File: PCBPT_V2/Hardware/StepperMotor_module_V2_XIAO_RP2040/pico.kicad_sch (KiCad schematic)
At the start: 12 parts, among them J2 External Ctrl, U1 MOUDLE-SEEEDUINO-XIAO

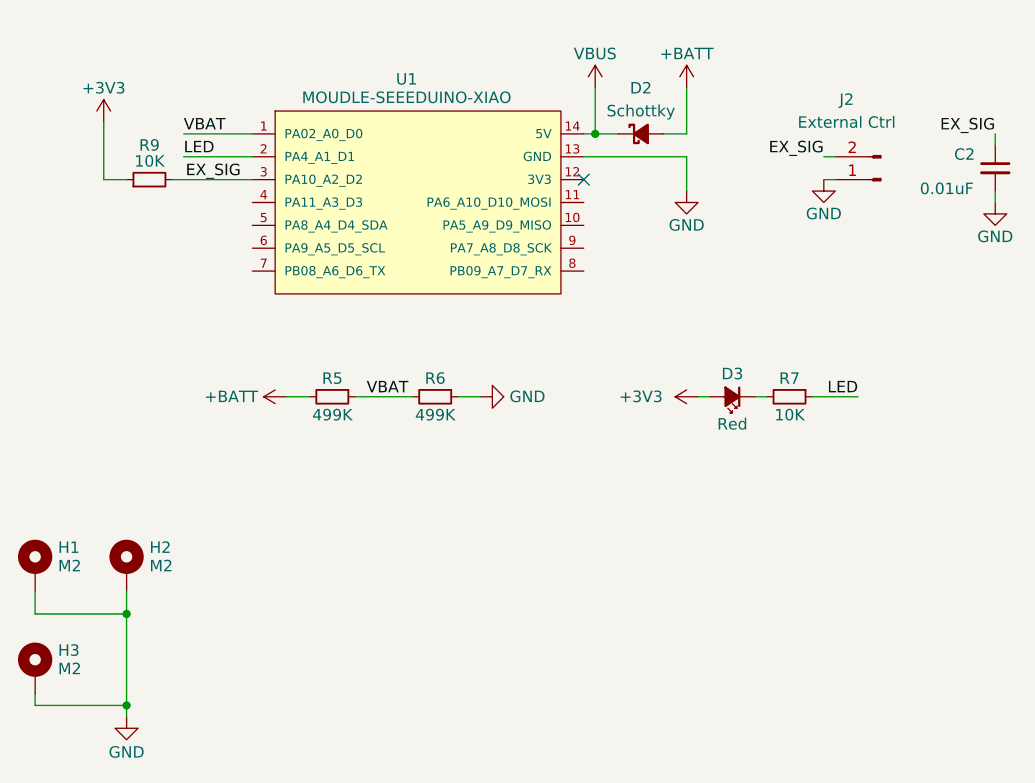
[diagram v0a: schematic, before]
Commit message: udated by FZ
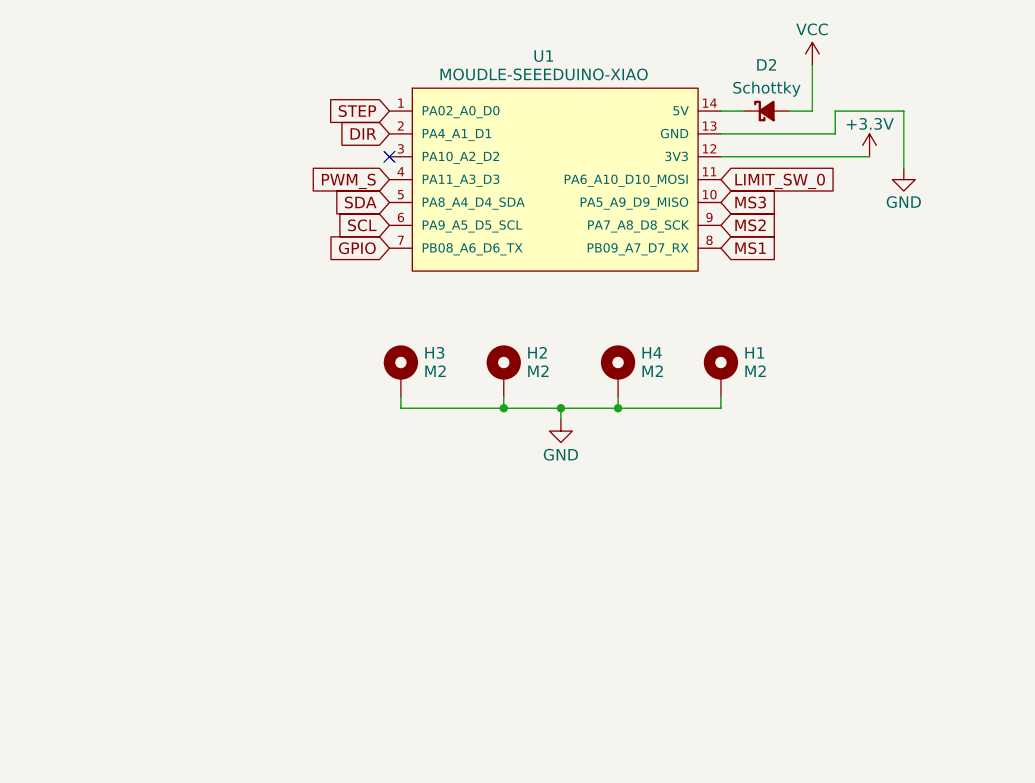
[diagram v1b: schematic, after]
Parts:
- removed C2: 0.01uF, Capacitor_SMD:C_0603_1608Metric_Pad1.08x0.95mm_HandSolder, symbol Device:C_Small
- removed D3: Red, LED_SMD:LED_0603_1608Metric_Pad1.05x0.95mm_HandSolder, symbol Device:LED_Small_Filled
- removed J2: External Ctrl, Connector_PinHeader_2.54mm:PinHeader_1x02_P2.54mm_Vertical, symbol Connector:Conn_01x02_Pin
- removed R5, R6: 499K, Resistor_SMD:R_0603_1608Metric_Pad0.98x0.95mm_HandSolder, symbol Device:R_Small
- removed R7, R9: 10K, Resistor_SMD:R_0603_1608Metric_Pad0.98x0.95mm_HandSolder, symbol Device:R_Small
- added H4: M2, MountingHole:MountingHole_2.2mm_M2_ISO7380_Pad, symbol Mechanical:MountingHole_Pad
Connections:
- net +3V3: now also U1.12 (3V3)
- net GND: now also H4.1
- net MS3: now reaches U1.10 (PA5_A9_D9_MISO)
- net LIMIT_SW_0: now reaches U1.11 (PA6_A10_D10_MOSI)
- net PWM_S: now reaches U1.4 (PA11_A3_D3)
- net SDA: now reaches U1.5 (PA8_A4_D4_SDA)
- net SCL: now reaches U1.6 (PA9_A5_D5_SCL)
- net GPIO: now reaches U1.7 (PB08_A6_D6_TX)
- net MS1: now reaches U1.8 (PB09_A7_D7_RX)
- net MS2: now reaches U1.9 (PA7_A8_D8_SCK)
- net +BATT renamed VCC
- net EX_SIG: no longer names the net of U1.3 (PA10_A2_D2)
- net LED renamed DIR
- net VBAT renamed STEP
- net VBUS: no longer names the net of D2.1 (K), U1.14 (5V)
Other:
- moved on the sheet: D2, H1, U1
